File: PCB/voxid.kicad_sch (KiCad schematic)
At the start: 58 parts, among them J1 Audio, J2 HPF_O, J3 LPFO, J4 Offset, J5 v3.3, J6 AudioOut, J7 v3.3, U1 TL072, U2 TL072, U3 TL072, U4 LM1117T-3.3

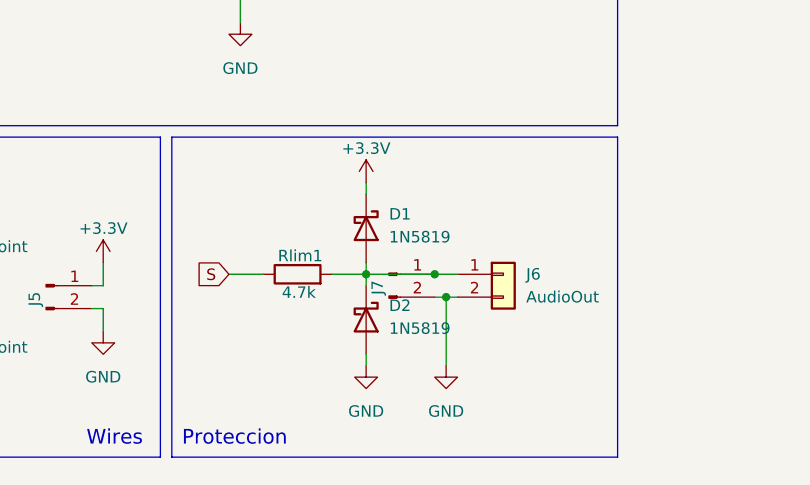
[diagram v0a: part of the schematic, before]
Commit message: pcb: Pcb lista :)
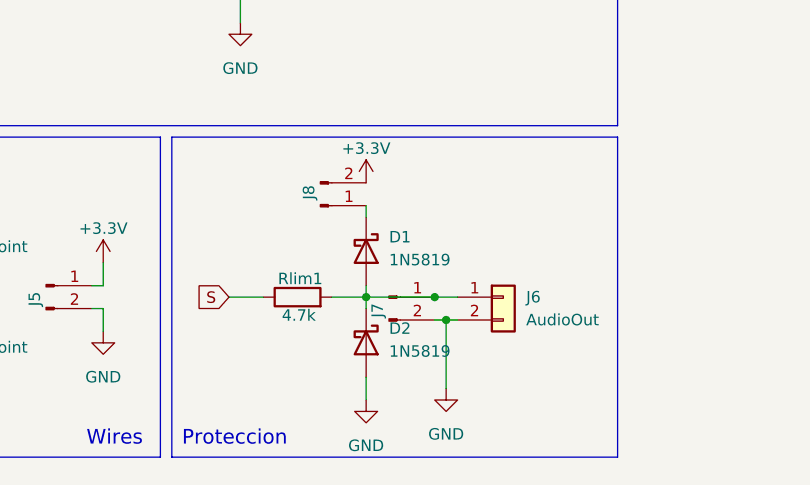
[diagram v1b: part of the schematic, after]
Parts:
- added J8: Offset, Connector_PinHeader_2.54mm:PinHeader_1x02_P2.54mm_Vertical, symbol Connector:Conn_01x02_Pin
- R1, R10, R14, R15, R16, R17, R18, R19, R2, R20, R21, R22, R23, R3, R4, R5, R6, Rlim1: footprint Resistor_THT:R_Axial_DIN0411_L9.9mm_D3.6mm_P12.70mm_Horizontal -> Resistor_THT:R_Axial_DIN0207_L6.3mm_D2.5mm_P7.62mm_Horizontal
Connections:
- net +3.3V: now also J8.2 (Pin_2); no longer D1.1 (K)
- new net: D1.1 (K), J8.1 (Pin_1)
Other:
- moved on the sheet: D1, D2, J6, J7, Rlim1
